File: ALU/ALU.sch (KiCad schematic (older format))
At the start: 40 parts, among them J1 Conn_01x16, J2 Conn_01x16, J3 Conn_01x08, J4 Conn_01x08, U1 74LS86, U10 74LS157, U11 74LS08, U12 74LS157, U13 74LS04, U2 74LS86, U3 74LS283, U4 74LS283, U5 74LS08, U6 74LS08, U7 74LS02, U8 74LS157, U9 74LS245

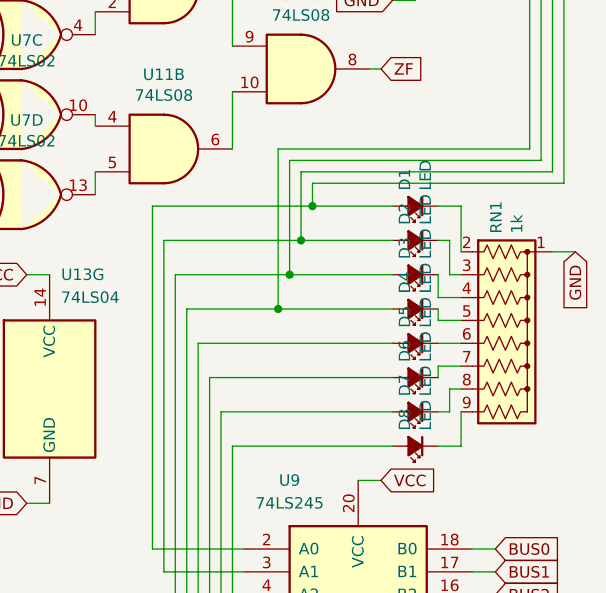
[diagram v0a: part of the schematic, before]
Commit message: Update all boards to r3, and update revision log and gitignore
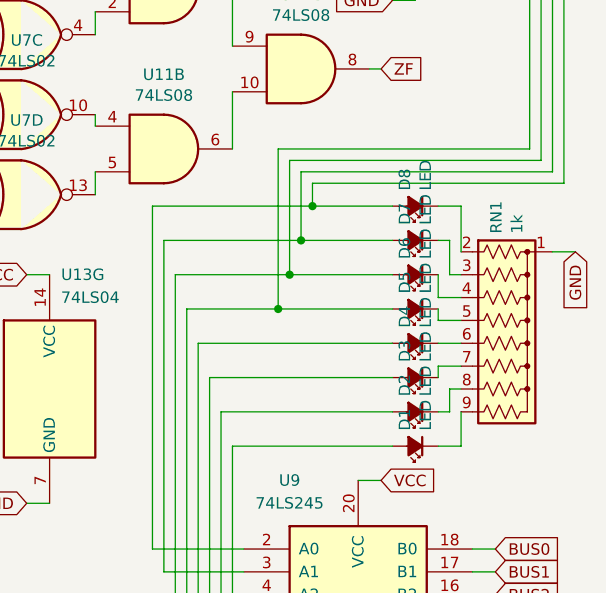
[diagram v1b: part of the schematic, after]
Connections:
- net at U12.4 (Za), U9.2 (A0): now also D8.2 (A); no longer D1.2 (A)
- net at U12.7 (Zb), U9.3 (A1): now also D7.2 (A); no longer D2.2 (A)
- net at U12.9 (Zc), U9.4 (A2): now also D6.2 (A); no longer D3.2 (A)
- net at U12.12 (Zd), U9.5 (A3): now also D5.2 (A); no longer D4.2 (A)
- net at U10.4 (Za), U7.8, U9.6 (A4): now also D4.2 (A); no longer D5.2 (A)
- net at U10.7 (Zb), U7.9, U9.7 (A5): now also D3.2 (A); no longer D6.2 (A)
- net at U10.9 (Zc), U7.11, U9.8 (A6): now also D2.2 (A); no longer D7.2 (A)
- net at U10.12 (Zd), U7.12, U9.9 (A7): now also D1.2 (A); no longer D8.2 (A)
- net at D1.1 (K): now also RN1.9 (R8); no longer RN1.2 (R1)
- net at D2.1 (K): now also RN1.8 (R7); no longer RN1.3 (R2)
- net at D3.1 (K): now also RN1.7 (R6); no longer RN1.4 (R3)
- net at D4.1 (K): now also RN1.6 (R5); no longer RN1.5 (R4)
- net at D5.1 (K): now also RN1.5 (R4); no longer RN1.6 (R5)
- net at D6.1 (K): now also RN1.4 (R3); no longer RN1.7 (R6)
- net at D7.1 (K): now also RN1.3 (R2); no longer RN1.8 (R7)
- net at D8.1 (K): now also RN1.2 (R1); no longer RN1.9 (R8)
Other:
- moved on the sheet: D1, D2, D3, D4, D5, D6, D7, D8
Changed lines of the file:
@@
 L Device:LED_Small_ALT D1
 U 1 1 5FA8CEA3
-P 10400 3350
-F 0 "D1" V 10446 3282 50  0000 R CNN
-F 1 "LED" V 10355 3282 50  0000 R CNN
-F 2 "LED_THT:LED_D3.0mm_Clear" V 10400 3350 50  0001 C CNN
-F 3 "~" V 10400 3350 50  0001 C CNN
-	1    10400 3350
+P 10400 4400
+F 0 "D1" V 10446 4332 50  0000 R CNN
+F 1 "LED" V 10355 4332 50  0000 R CNN
+F 2 "LED_THT:LED_D3.0mm_Clear" V 10400 4400 50  0001 C CNN
+F 3 "~" V 10400 4400 50  0001 C CNN
+	1    10400 4400
 	-1   0    0    1
 $EndComp
@@
 L Device:LED_Small_ALT D2
 U 1 1 5FA9128B
+P 10400 4250
+F 0 "D2" V 10446 4182 50  0000 R CNN
+F 1 "LED" V 10355 4182 50  0000 R CNN
+F 2 "LED_THT:LED_D3.0mm_Clear" V 10400 4250 50  0001 C CNN
+F 3 "~" V 10400 4250 50  0001 C CNN
+	1    10400 4250
+	-1   0    0    1
+$EndComp
+$Comp
+L Device:LED_Small_ALT D3
+U 1 1 5FA9DF77
+P 10400 4100
+F 0 "D3" V 10446 4032 50  0000 R CNN
+F 1 "LED" V 10355 4032 50  0000 R CNN
+F 2 "LED_THT:LED_D3.0mm_Clear" V 10400 4100 50  0001 C CNN
+F 3 "~" V 10400 4100 50  0001 C CNN
+	1    10400 4100
+	-1   0    0    1
+$EndComp
+$Comp
+L Device:LED_Small_ALT D4
+U 1 1 5FAAAACD
+P 10400 3950
+F 0 "D4" V 10446 3882 50  0000 R CNN
+F 1 "LED" V 10355 3882 50  0000 R CNN
+F 2 "LED_THT:LED_D3.0mm_Clear" V 10400 3950 50  0001 C CNN
+F 3 "~" V 10400 3950 50  0001 C CNN
+	1    10400 3950
+	-1   0    0    1
+$EndComp
+$Comp
+L Device:LED_Small_ALT D5
+U 1 1 5FAB9D8B
+P 10400 3800
+F 0 "D5" V 10446 3732 50  0000 R CNN
+F 1 "LED" V 10355 3732 50  0000 R CNN
+F 2 "LED_THT:LED_D3.0mm_Clear" V 10400 3800 50  0001 C CNN
+F 3 "~" V 10400 3800 50  0001 C CNN
+	1    10400 3800
+	-1   0    0    1
+$EndComp
+$Comp
+L Device:LED_Small_ALT D6
+U 1 1 5FAB9D91
+P 10400 3650
+F 0 "D6" V 10446 3582 50  0000 R CNN
+F 1 "LED" V 10355 3582 50  0000 R CNN
+F 2 "LED_THT:LED_D3.0mm_Clear" V 10400 3650 50  0001 C CNN
+F 3 "~" V 10400 3650 50  0001 C CNN
+	1    10400 3650
+	-1   0    0    1
+$EndComp
+$Comp
+L Device:LED_Small_ALT D7
+U 1 1 5FAB9D97
 P 10400 3500
-F 0 "D2" V 10446 3432 50  0000 R CNN
+F 0 "D7" V 10446 3432 50  0000 R CNN
 F 1 "LED" V 10355 3432 50  0000 R CNN
 F 2 "LED_THT:LED_D3.0mm_Clear" V 10400 3500 50  0001 C CNN
@@
 $EndComp
 $Comp
-L Device:LED_Small_ALT D3
-U 1 1 5FA9DF77
-P 10400 3650
-F 0 "D3" V 10446 3582 50  0000 R CNN
-F 1 "LED" V 10355 3582 50  0000 R CNN
-F 2 "LED_THT:LED_D3.0mm_Clear" V 10400 3650 50  0001 C CNN
-F 3 "~" V 10400 3650 50  0001 C CNN
-	1    10400 3650
+L Device:LED_Small_ALT D8
+U 1 1 5FAB9D9D
+P 10400 3350
+F 0 "D8" V 10446 3282 50  0000 R CNN
+F 1 "LED" V 10355 3282 50  0000 R CNN
+F 2 "LED_THT:LED_D3.0mm_Clear" V 10400 3350 50  0001 C CNN
+F 3 "~" V 10400 3350 50  0001 C CNN
+	1    10400 3350
 	-1   0    0    1
 $EndComp
-$Comp
-L Device:LED_Small_ALT D4
-U 1 1 5FAAAACD
-P 10400 3800
-F 0 "D4" V 10446 3732 50  0000 R CNN
-F 1 "LED" V 10355 3732 50  0000 R CNN
-F 2 "LED_THT:LED_D3.0mm_Clear" V 10400 3800 50  0001 C CNN
-F 3 "~" V 10400 3800 50  0001 C CNN
-	1    10400 3800
-	-1   0    0    1
-$EndComp
-$Comp
-L Device:LED_Small_ALT D5
-U 1 1 5FAB9D8B
-P 10400 3950
-F 0 "D5" V 10446 3882 50  0000 R CNN
-F 1 "LED" V 10355 3882 50  0000 R CNN
-F 2 "LED_THT:LED_D3.0mm_Clear" V 10400 3950 50  0001 C CNN
-F 3 "~" V 10400 3950 50  0001 C CNN
-	1    10400 3950
-	-1   0    0    1
-$EndComp
-$Comp
-L Device:LED_Small_ALT D6
-U 1 1 5FAB9D91
-P 10400 4100
-F 0 "D6" V 10446 4032 50  0000 R CNN
-F 1 "LED" V 10355 4032 50  0000 R CNN
-F 2 "LED_THT:LED_D3.0mm_Clear" V 10400 4100 50  0001 C CNN
-F 3 "~" V 10400 4100 50  0001 C CNN
-	1    10400 4100
-	-1   0    0    1
-$EndComp
-$Comp
-L Device:LED_Small_ALT D7
-U 1 1 5FAB9D97
-P 10400 4250
-F 0 "D7" V 10446 4182 50  0000 R CNN
-F 1 "LED" V 10355 4182 50  0000 R CNN
-F 2 "LED_THT:LED_D3.0mm_Clear" V 10400 4250 50  0001 C CNN
-F 3 "~" V 10400 4250 50  0001 C CNN
-	1    10400 4250
-	-1   0    0    1
-$EndComp
-$Comp
-L Device:LED_Small_ALT D8
-U 1 1 5FAB9D9D
-P 10400 4400
-F 0 "D8" V 10446 4332 50  0000 R CNN
-F 1 "LED" V 10355 4332 50  0000 R CNN
-F 2 "LED_THT:LED_D3.0mm_Clear" V 10400 4400 50  0001 C CNN
-F 3 "~" V 10400 4400 50  0001 C CNN
-	1    10400 4400
-	-1   0    0    1
-$EndComp
